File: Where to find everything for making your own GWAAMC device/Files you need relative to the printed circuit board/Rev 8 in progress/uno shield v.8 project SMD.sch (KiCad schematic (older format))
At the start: 108 parts, among them J1 Conn_3.5mm, J2 Power, J3 Analog, J4 Digital, J5 Digital, J6 Conn_01x09_Female, J6_A7,A6 Conn_01x02_gender_unknown, J7_A7,A6 Conn_01x02_Female, J9 TE_1-2328702-0, P1 CONN_01X01, P2 CONN_01X01, P3 CONN_01X01, P4 CONN_01X01, Q1 MMBF5460 (2N5460), Q2 MMBF5460 (2N5460), Q3 DMN601K-7, Q4 DMN601K-7, Q5 DMN601K-7, Q6 DMN601K-7, Q7 DMN601K-7, U1 3V LDO, U10 MCP4262-502E/UN, U11 MCP4262-502E/UN, U12 MCP4262-502E/UN, U13 MCP4262-502E/UN, U14 MCP4262-502E/UN, U15 MCP4262-502E/UN, U16 MCP4262-502E/UN, U17 MCP4262-502E/UN, U18 MCP4262-502E/UN, U19 MCP4262-502E/UN, U2 AD8244ARMZ, U20 MCP4262-502E/UN, U21 MCP4262-502E/UN, U22 MCP4262-502E/UN, U23 MCP4262-502E/UN, U24 MCP4262-502E/UN, U25 MCP4262-502E/UN, U26 MCP4262-502E/UN, U27 MCP4262-502E/UN, U28 MCP4262-502E/UN, U29 MCP4262-502E/UN, U3 ADL5315ACPZ-R7, U30 MCP4262-502E/UN, U31 MCP4262-502E/UN, U32 MCP4262-502E/UN, U33 MCP4262-502E/UN, U4 REF200AU, U5 LM334M, U6 LM334M, U7 MCP4262-503E/UN, U8 - U32 all in parallel MCP4262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, U9 MCP4262-502E/UN

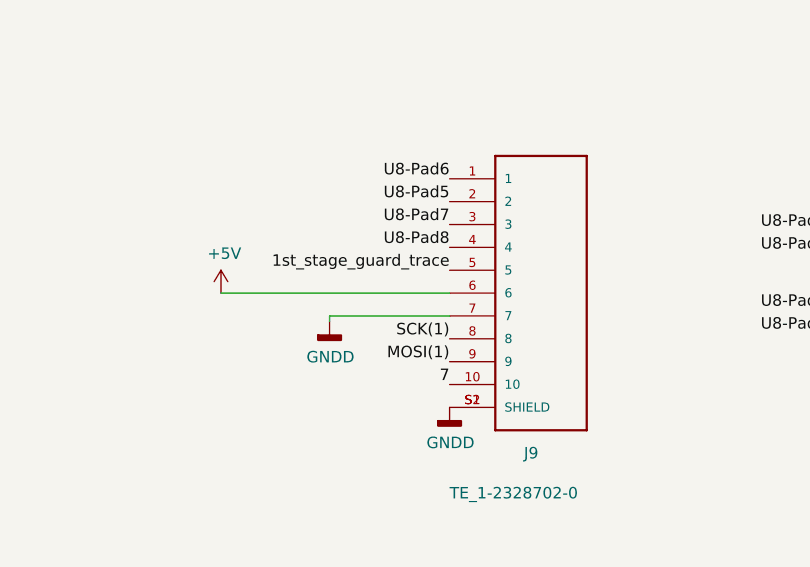
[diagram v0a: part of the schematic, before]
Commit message: In the latest state of progress...
...definitely not in working state, but where I'll resume work when I get back to things.
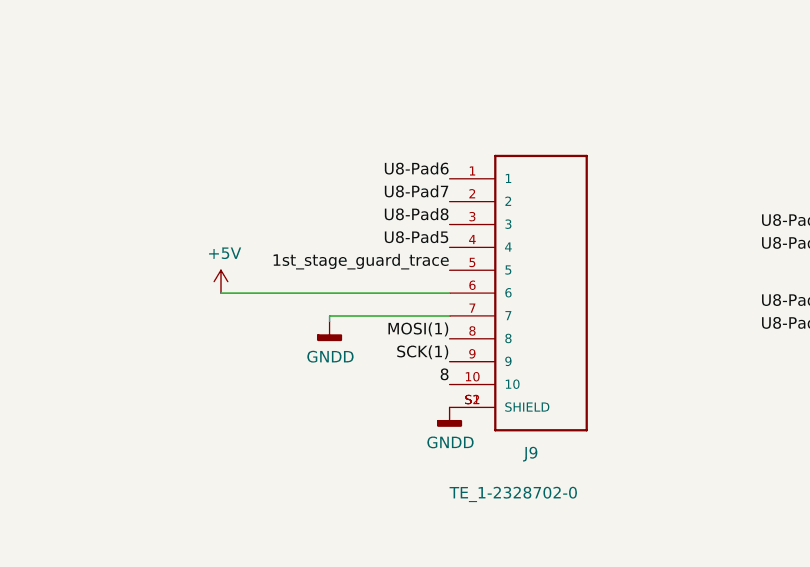
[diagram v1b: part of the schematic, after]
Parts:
- J9: Source https://www.te.com/ OR http://Arrow.com (factory direct can actually be a few cents cheaper!) -> https://www.te.com/ OR http://Arrow.com (factory direct can actually be a few cents cheaper with this one!)
- U10, U11, U12, U13, U14, U15, U16, U17, U18, U19, U20, U21, U22, U23, U24, U25, U26, U27, U28, U29, U30, U31, U32, U33, U9: ClickToSortForPlacement 15 NOT ACCOMMODATED ON BOARD REV 7 AND BELOW: PATCHING IN R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 -> 15 NOT WELL ACCOMMODATED ON BOARD REV 7 AND BELOW: PATCHING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
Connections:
- net 7: no longer J9.10
- net 8: now also J9.10
- net MOSI(1): now also J9.8; no longer J9.9
- net SCK(1): now also J9.9; no longer J9.8
- net U8-Pad5: now also J9.4; no longer J9.2
- net U8-Pad7: now also J9.2; no longer J9.3
- net U8-Pad8: now also J9.3; no longer J9.4

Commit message: In the latest state of progress...
...definitely not in working state, but where I'll resume work when I get back to things.
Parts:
- ADC1: symbol newkicadversion-rescue:HX711-hx711 -> uno-shield-v.8-project-SMD-rescue:HX711-hx711-newkicadversion-rescue
- J1: symbol audiojack3_ground_switchtr:AudioJack3_Ground_SwitchTR -> uno-shield-v.8-project-SMD-rescue:AudioJack3_Ground_SwitchTR-audiojack3_ground_switchtr
- J3: symbol conn_01x06_male:Conn_01x06_Male -> uno-shield-v.8-project-SMD-rescue:Conn_01x06_Male-conn_01x06_male
- J5: symbol conn_01x08_maleA:Conn_01x08_Male -> uno-shield-v.8-project-SMD-rescue:Conn_01x08_Male-conn_01x08_maleA
- J9: symbol 1-2328702-0:1-2328702-0 -> uno-shield-v.8-project-SMD-rescue:1-2328702-0-1-2328702-0
- JP10, JP11, JP8, JP9: symbol solderjumper_3_bridged12:SolderJumper_3_Bridged12 -> uno-shield-v.8-project-SMD-rescue:SolderJumper_3_Bridged12-solderjumper_3_bridged12
- U10, U11, U12, U13, U14, U15, U16, U17, U18, U19, U20, U21, U22, U23, U24, U25, U26, U27, U28, U29, U30, U31, U32, U33, U7, U8, U9: symbol 2019-03-19_09-09-09:MCP4262-xxxE_UN -> uno-shield-v.8-project-SMD-rescue:MCP4262-xxxE_UN-2019-03-19_09-09-09
- U2: symbol newkicadversion-rescue:AD8244ARMZ-AD8244_A -> uno-shield-v.8-project-SMD-rescue:AD8244ARMZ-AD8244_A-newkicadversion-rescue
- U3: symbol uno-shield-rescue:ADL5315ACPZ-R7-2019-05-19_00-44-38-uno-shield-rescue-uno-shield-rescue -> uno-shield-v.8-project-SMD-rescue:ADL5315ACPZ-R7-2019-05-19_00-44-38-uno-shield-rescue-uno-shield-rescue-uno-shield-res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
- U4: symbol Reference_Current:REF200AU -> uno-shield-v.8-project-SMD-rescue:REF200AU-Reference_Current
- U5, U6: symbol lm334m:LM334M -> uno-shield-v.8-project-SMD-rescue:LM334M-lm334m
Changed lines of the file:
@@
 Connection ~ 3575 5450
 $Comp
-L audiojack3_ground_switchtr:AudioJack3_Ground_SwitchTR J1
+L uno-shield-v.8-project-SMD-rescue:AudioJack3_Ground_SwitchTR-audiojack3_ground_switchtr J1
 U 1 1 5C536746
 P 1500 4800
@@
 $EndComp
 $Comp
-L newkicadversion-rescue:AD8244ARMZ-AD8244_A U2
+L uno-shield-v.8-project-SMD-rescue:AD8244ARMZ-AD8244_A-newkicadversion-rescue U2
 U 4 1 5C72CF84
 P 12800 6400
@@
 $EndComp
 $Comp
-L conn_01x08_maleA:Conn_01x08_Male J5
+L uno-shield-v.8-project-SMD-rescue:Conn_01x08_Male-conn_01x08_maleA J5
 U 1 1 5C8A7B72
 P 21850 2500
@@
 $EndComp
 $Comp
-L conn_01x06_male:Conn_01x06_Male J3
+L uno-shield-v.8-project-SMD-rescue:Conn_01x06_Male-conn_01x06_male J3
 U 1 1 5C90EA9D
 P 21250 2400
@@
 $EndComp
 $Comp
-L newkicadversion-rescue:AD8244ARMZ-AD8244_A U2
+L uno-shield-v.8-project-SMD-rescue:AD8244ARMZ-AD8244_A-newkicadversion-rescue U2
 U 2 1 5F04F6CF
 P 12800 4775
@@
 $EndComp
 $Comp
-L newkicadversion-rescue:HX711-hx711 ADC1
+L uno-shield-v.8-project-SMD-rescue:HX711-hx711-newkicadversion-rescue ADC1
 U 1 1 5C19811F
 P 15350 5100
@@
 $EndComp
 $Comp
-L newkicadversion-rescue:AD8244ARMZ-AD8244_A U2
+L uno-shield-v.8-project-SMD-rescue:AD8244ARMZ-AD8244_A-newkicadversion-rescue U2
 U 1 1 5F04DF16
 P 12800 4150
@@
 $EndComp
 $Comp
-L Reference_Current:REF200AU U4
+L uno-shield-v.8-project-SMD-rescue:REF200AU-Reference_Current U4
 U 3 1 5D0FCC87
 P 7775 5150
@@
 $EndComp
 $Comp
-L Reference_Current:REF200AU U4
+L uno-shield-v.8-project-SMD-rescue:REF200AU-Reference_Current U4
 U 2 1 5D0FB910
 P 8375 6000
@@
 $EndComp
 $Comp
-L uno-shield-rescue:ADL5315ACPZ-R7-2019-05-19_00-44-38-uno-shield-rescue-uno-shield-rescue U3
+L uno-shield-v.8-project-SMD-rescue:ADL5315ACPZ-R7-2019-05-19_00-44-38-uno-shield-rescue-uno-shield-rescue-uno-shield-rescue U3
 U 1 1 5CE2F217
 P 3800 4650
@@
 $EndComp
 $Comp
-L 2019-03-19_09-09-09:MCP4262-xxxE_UN U8
+L uno-shield-v.8-project-SMD-rescue:MCP4262-xxxE_UN-2019-03-19_09-09-09 U8
 U 1 1 5CA59032
 P 11100 4575
@@
 $EndComp
 $Comp
-L lm334m:LM334M U5
+L uno-shield-v.8-project-SMD-rescue:LM334M-lm334m U5
 U 1 1 5CDCE965
 P 7775 3950
@@
 $EndComp
 $Comp
-L lm334m:LM334M U6
+L uno-shield-v.8-project-SMD-rescue:LM334M-lm334m U6
 U 1 1 5CDCF5D4
 P 8875 3950
@@
 $EndComp
 $Comp
-L newkicadversion-rescue:AD8244ARMZ-AD8244_A U2
+L uno-shield-v.8-project-SMD-rescue:AD8244ARMZ-AD8244_A-newkicadversion-rescue U2
 U 3 1 5F050747
 P 3450 4075
@@
 $EndComp
 $Comp
-L solderjumper_3_bridged12:SolderJumper_3_Bridged12 JP8
+L uno-shield-v.8-project-SMD-rescue:SolderJumper_3_Bridged12-solderjumper_3_bridged12 JP8
 U 1 1 5D438593
 P 17700 9075
@@
 $EndComp
 $Comp
-L solderjumper_3_bridged12:SolderJumper_3_Bridged12 JP10
+L uno-shield-v.8-project-SMD-rescue:SolderJumper_3_Bridged12-solderjumper_3_bridged12 JP10
 U 1 1 5D43B289
 P 18400 8975
@@
 $EndComp
 $Comp
-L solderjumper_3_bridged12:SolderJumper_3_Bridged12 JP11
+L uno-shield-v.8-project-SMD-rescue:SolderJumper_3_Bridged12-solderjumper_3_bridged12 JP11
 U 1 1 5D43C8EF
 P 18400 9575
@@
 $EndComp
 $Comp
-L solderjumper_3_bridged12:SolderJumper_3_Bridged12 JP9
+L uno-shield-v.8-project-SMD-rescue:SolderJumper_3_Bridged12-solderjumper_3_bridged12 JP9
 U 1 1 5D43D9B5
 P 17700 9675
@@
 $EndComp
 $Comp
-L 2019-03-19_09-09-09:MCP4262-xxxE_UN U12
+L uno-shield-v.8-project-SMD-rescue:MCP4262-xxxE_UN-2019-03-19_09-09-09 U12
 U 1 1 5D6AAC30
 P 6950 -825
@@
 $EndComp
 $Comp
-L 2019-03-19_09-09-09:MCP4262-xxxE_UN U16
+L uno-shield-v.8-project-SMD-rescue:MCP4262-xxxE_UN-2019-03-19_09-09-09 U16
 U 1 1 5D79DE00
 P 8725 -775
@@
 $EndComp
 $Comp
-L 2019-03-19_09-09-09:MCP4262-xxxE_UN U20
+L uno-shield-v.8-project-SMD-rescue:MCP4262-xxxE_UN-2019-03-19_09-09-09 U20
 U 1 1 5D7B7390
 P 10325 -800
@@
 $EndComp
 $Comp
-L 2019-03-19_09-09-09:MCP4262-xxxE_UN U24
+L uno-shield-v.8-project-SMD-rescue:MCP4262-xxxE_UN-2019-03-19_09-09-09 U24
 U 1 1 5D7D0E54
 P 11950 -775
@@
 $EndComp
 $Comp
-L 2019-03-19_09-09-09:MCP4262-xxxE_UN U28
+L uno-shield-v.8-project-SMD-rescue:MCP4262-xxxE_UN-2019-03-19_09-09-09 U28
 U 1 1 5D7E9C86
 P 13700 -750
@@
 $EndComp
 $Comp
-L 2019-03-19_09-09-09:MCP4262-xxxE_UN U32
+L uno-shield-v.8-project-SMD-rescue:MCP4262-xxxE_UN-2019-03-19_09-09-09 U32
 U 1 1 5D8038A3
 P 15225 -750
@@
 $EndComp
 $Comp
-L 2019-03-19_09-09-09:MCP4262-xxxE_UN U11
+L uno-shield-v.8-project-SMD-rescue:MCP4262-xxxE_UN-2019-03-19_09-09-09 U11
 U 1 1 5D88DEC2
 P 6900 -2500
@@
 $EndComp
 $Comp
-L 2019-03-19_09-09-09:MCP4262-xxxE_UN U15
+L uno-shield-v.8-project-SMD-rescue:MCP4262-xxxE_UN-2019-03-19_09-09-09 U15
 U 1 1 5D88DEE1
 P 8675 -2450
@@
 $EndComp
 $Comp
-L 2019-03-19_09-09-09:MCP4262-xxxE_UN U19
+L uno-shield-v.8-project-SMD-rescue:MCP4262-xxxE_UN-2019-03-19_09-09-09 U19
 U 1 1 5D88DF00
 P 10275 -2475
@@
 $EndComp
 $Comp
-L 2019-03-19_09-09-09:MCP4262-xxxE_UN U23
+L uno-shield-v.8-project-SMD-rescue:MCP4262-xxxE_UN-2019-03-19_09-09-09 U23
 U 1 1 5D88DF1F
 P 11900 -2450
@@
 $EndComp
 $Comp
-L 2019-03-19_09-09-09:MCP4262-xxxE_UN U27
+L uno-shield-v.8-project-SMD-rescue:MCP4262-xxxE_UN-2019-03-19_09-09-09 U27
 U 1 1 5D88DF3E
 P 13650 -2425
@@
 $EndComp
 $Comp
-L 2019-03-19_09-09-09:MCP4262-xxxE_UN U31
+L uno-shield-v.8-project-SMD-rescue:MCP4262-xxxE_UN-2019-03-19_09-09-09 U31
 U 1 1 5D88DF5D
 P 15175 -2425
@@
 $EndComp
 $Comp
-L 2019-03-19_09-09-09:MCP4262-xxxE_UN U10
+L uno-shield-v.8-project-SMD-rescue:MCP4262-xxxE_UN-2019-03-19_09-09-09 U10
 U 1 1 5D8ACEF1
 P 6875 -4325
@@
 $EndComp
 $Comp
-L 2019-03-19_09-09-09:MCP4262-xxxE_UN U14
+L uno-shield-v.8-project-SMD-rescue:MCP4262-xxxE_UN-2019-03-19_09-09-09 U14
 U 1 1 5D8ACF10
 P 8650 -4275
@@
 $EndComp
 $Comp
-L 2019-03-19_09-09-09:MCP4262-xxxE_UN U18
+L uno-shield-v.8-project-SMD-rescue:MCP4262-xxxE_UN-2019-03-19_09-09-09 U18
 U 1 1 5D8ACF2F
 P 10250 -4300
@@
 $EndComp
 $Comp
-L 2019-03-19_09-09-09:MCP4262-xxxE_UN U22
+L uno-shield-v.8-project-SMD-rescue:MCP4262-xxxE_UN-2019-03-19_09-09-09 U22
 U 1 1 5D8ACF4E
 P 11875 -4275
@@
 $EndComp
 $Comp
-L 2019-03-19_09-09-09:MCP4262-xxxE_UN U26
+L uno-shield-v.8-project-SMD-rescue:MCP4262-xxxE_UN-2019-03-19_09-09-09 U26
 U 1 1 5D8ACF6D
 P 13625 -4250
@@
 $EndComp
 $Comp
-L 2019-03-19_09-09-09:MCP4262-xxxE_UN U30
+L uno-shield-v.8-project-SMD-rescue:MCP4262-xxxE_UN-2019-03-19_09-09-09 U30
 U 1 1 5D8ACF8C
 P 15150 -4250
@@
 $EndComp
 $Comp
-L 2019-03-19_09-09-09:MCP4262-xxxE_UN U9
+L uno-shield-v.8-project-SMD-rescue:MCP4262-xxxE_UN-2019-03-19_09-09-09 U9
 U 1 1 5D8CCF9E
 P 6850 -6150
@@
 $EndComp
 $Comp
-L 2019-03-19_09-09-09:MCP4262-xxxE_UN U13
+L uno-shield-v.8-project-SMD-rescue:MCP4262-xxxE_UN-2019-03-19_09-09-09 U13
 U 1 1 5D8CCFBD
 P 8625 -6100
@@
 $EndComp
 $Comp
-L 2019-03-19_09-09-09:MCP4262-xxxE_UN U17
+L uno-shield-v.8-project-SMD-rescue:MCP4262-xxxE_UN-2019-03-19_09-09-09 U17
 U 1 1 5D8CCFDC
 P 10225 -6125
@@
 $EndComp
 $Comp
-L 2019-03-19_09-09-09:MCP4262-xxxE_UN U21
+L uno-shield-v.8-project-SMD-rescue:MCP4262-xxxE_UN-2019-03-19_09-09-09 U21
 U 1 1 5D8CCFFB
 P 11850 -6100
@@
 $EndComp
 $Comp
-L 2019-03-19_09-09-09:MCP4262-xxxE_UN U25
+L uno-shield-v.8-project-SMD-rescue:MCP4262-xxxE_UN-2019-03-19_09-09-09 U25
 U 1 1 5D8CD01A
 P 13600 -6075
@@
 $EndComp
 $Comp
-L 2019-03-19_09-09-09:MCP4262-xxxE_UN U29
+L uno-shield-v.8-project-SMD-rescue:MCP4262-xxxE_UN-2019-03-19_09-09-09 U29
 U 1 1 5D8CD039
 P 15125 -6075
@@
 $EndComp
 $Comp
-L 2019-03-19_09-09-09:MCP4262-xxxE_UN U33
+L uno-shield-v.8-project-SMD-rescue:MCP4262-xxxE_UN-2019-03-19_09-09-09 U33
 U 1 1 5D8EC9A4
 P 16975 -725
@@
 U8-Pad5
 $Comp
-L 2019-03-19_09-09-09:MCP4262-xxxE_UN U7
+L uno-shield-v.8-project-SMD-rescue:MCP4262-xxxE_UN-2019-03-19_09-09-09 U7
 U 1 1 5C9A2EF5
 P 9850 4575
@@
 	9525 4025 9525 4275
 $Comp
-L 1-2328702-0:1-2328702-0 J9
+L uno-shield-v.8-project-SMD-rescue:1-2328702-0-1-2328702-0 J9
 U 1 1 5DA5E558
 P 5350 -800
@@
 1st_stage_guard_trace
 $Comp
-L Reference_Current:REF200AU U4
+L uno-shield-v.8-project-SMD-rescue:REF200AU-Reference_Current U4
 U 1 1 5D0F9980
 P 6150 3525
